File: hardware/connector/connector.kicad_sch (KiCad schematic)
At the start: 16 parts, among them J1 Conn_02x28_Top_Bottom, J2 D38999

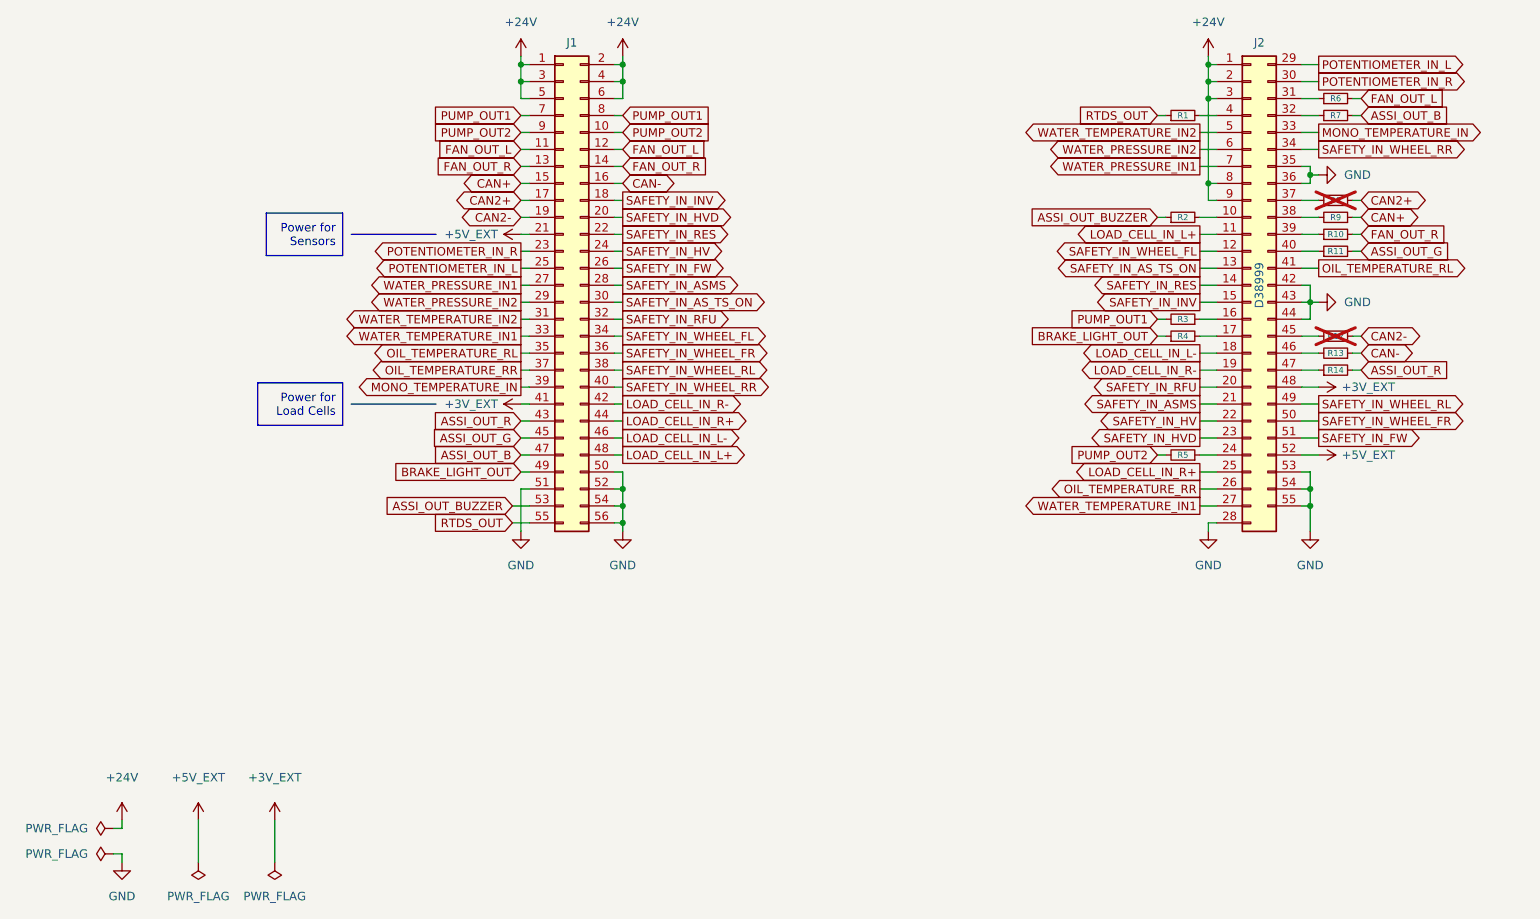
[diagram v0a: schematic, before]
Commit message: Sync :(
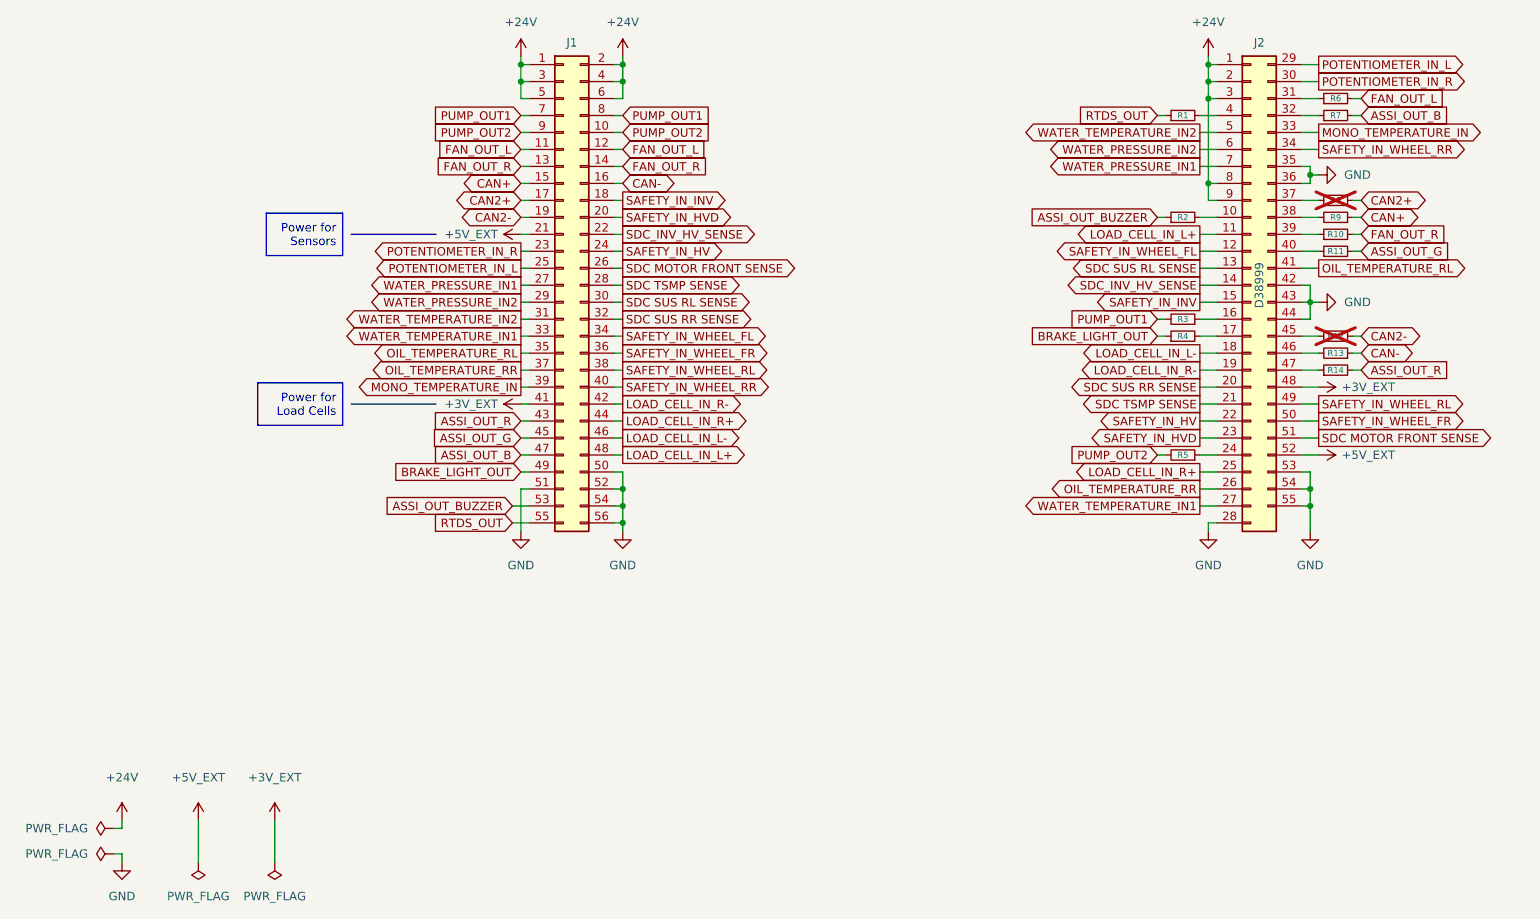
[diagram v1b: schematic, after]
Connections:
- net SAFETY_IN_ASMS renamed SDC TSMP SENSE
- net SAFETY_IN_AS_TS_ON renamed  SDC SUS RL SENSE
- net SAFETY_IN_FW renamed SDC MOTOR FRONT SENSE
- net SAFETY_IN_RES renamed SDC_INV_HV_SENSE
- net SAFETY_IN_RFU renamed  SDC SUS RR SENSE
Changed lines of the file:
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@@
 (kicad_sch
-	(version 20231120)
+	(version 20250114)
 	(generator "eeschema")
-	(generator_version "8.0")
+	(generator_version "9.0")
 	(paper "A4")
 	(title_block
@@
 		(comment 1 "Reviewer:")
 	)
+	(text_box "Power for Sensors"
+		(exclude_from_sim no)
+		(at 59.69 86.995 0)
+		(size 11.43 6.35)
+		(margins 0.9525 0.9525 0.9525 0.9525)
+		(stroke
+			(width 0)
+			(type default)
+		)
+		(fill
+			(type none)
+		)
+		(effects
+			(font
+				(size 1.27 1.27)
+			)
+			(justify right)
+		)
+	)
+	(text_box "Power for Load Cells"
+		(exclude_from_sim no)
+		(at 58.42 112.395 0)
+		(size 12.7 6.35)
+		(margins 0.9525 0.9525 0.9525 0.9525)
+		(stroke
+			(width 0)
+			(type default)
+		)
+		(fill
+			(type none)
+		)
+		(effects
+			(font
+				(size 1.27 1.27)
+			)
+			(justify right)
+		)
+	)
 	(junction
 		(at 113.03 64.77)
@@
 		)
 	)
-	(text_box "Power for Sensors"
-		(exclude_from_sim no)
-		(at 59.69 86.995 0)
-		(size 11.43 6.35)
-		(stroke
-			(width 0)
-			(type default)
-		)
-		(fill
-			(type none)
-		)
-		(effects
-			(font
-				(size 1.27 1.27)
-			)
-			(justify right)
-		)
-	)
-	(text_box "Power for Load Cells"
-		(exclude_from_sim no)
-		(at 58.42 112.395 0)
-		(size 12.7 6.35)
-		(stroke
-			(width 0)
-			(type default)
-		)
-		(fill
-			(type none)
-		)
-		(effects
-			(font
-				(size 1.27 1.27)
-			)
-			(justify right)
-		)
-	)
-	(global_label "SAFETY_IN_RFU"
+	(global_label " SDC SUS RR SENSE"
 		(shape output)
 		(at 113.03 102.87 0)
@@
 		)
 		(property "Intersheetrefs" "${INTERSHEET_REFS}"
-			(at 130.1667 102.87 0)
+			(at 135.9721 102.87 0)
 			(effects
 				(font
@@
 		)
 	)
-	(global_label "SAFETY_IN_ASMS"
+	(global_label "SDC TSMP SENSE"
 		(shape output)
 		(at 199.39 115.57 180)
@@
 		)
 		(property "Intersheetrefs" "${INTERSHEET_REFS}"
-			(at 181.0628 115.57 0)
+			(at 179.7741 115.57 0)
 			(effects
 				(font
@@
 		)
 	)
-	(global_label "SAFETY_IN_AS_TS_ON"
+	(global_label " SDC SUS RL SENSE"
 		(shape output)
 		(at 199.39 95.25 180)
@@
 		)
 		(property "Intersheetrefs" "${INTERSHEET_REFS}"
-			(at 176.871 95.25 0)
+			(at 176.6898 95.25 0)
 			(effects
 				(font
@@
 		)
 	)
-	(global_label "SAFETY_IN_FW"
+	(global_label "SDC MOTOR FRONT SENSE"
 		(shape output)
 		(at 217.17 120.65 0)
@@
 		)
 		(property "Intersheetrefs" "${INTERSHEET_REFS}"
-			(at 233.1576 120.65 0)
+			(at 245.1922 120.65 0)
 			(effects
 				(font
@@
 		)
 	)
-	(global_label "SAFETY_IN_RES"
+	(global_label "SDC_INV_HV_SENSE"
 		(shape output)
 		(at 113.03 90.17 0)
@@
 		)
 		(property "Intersheetrefs" "${INTERSHEET_REFS}"
-			(at 130.0267 90.17 0)
+			(at 134.158 90.17 0)
 			(effects
 				(font
@@
 		)
 	)
-	(global_label "SAFETY_IN_RFU"
+	(global_label " SDC SUS RR SENSE"
 		(shape output)
 		(at 199.39 113.03 180)
@@
 		)
 		(property "Intersheetrefs" "${INTERSHEET_REFS}"
-			(at 182.2533 113.03 0)
+			(at 176.4479 113.03 0)
 			(effects
 				(font
@@
 		)
 	)
-	(global_label "SAFETY_IN_RES"
+	(global_label "SDC_INV_HV_SENSE"
 		(shape output)
 		(at 199.39 97.79 180)
@@
 		)
 		(property "Intersheetrefs" "${INTERSHEET_REFS}"
-			(at 182.3933 97.79 0)
+			(at 178.262 97.79 0)
 			(effects
 				(font
@@
 		)
 	)
-	(global_label "SAFETY_IN_ASMS"
+	(global_label "SDC TSMP SENSE"
 		(shape output)
 		(at 113.03 97.79 0)
@@
 		)
 		(property "Intersheetrefs" "${INTERSHEET_REFS}"
-			(at 131.3572 97.79 0)
+			(at 132.6459 97.79 0)
 			(effects
 				(font
@@
 		)
 	)
-	(global_label "SAFETY_IN_FW"
+	(global_label "SDC MOTOR FRONT SENSE"
 		(shape output)
 		(at 113.03 95.25 0)
@@
 		)
 		(property "Intersheetrefs" "${INTERSHEET_REFS}"
-			(at 128.9382 95.25 0)
+			(at 141.0522 95.25 0)
 			(effects
 				(font
@@
 		)
 	)
-	(global_label "SAFETY_IN_AS_TS_ON"
+	(global_label " SDC SUS RL SENSE"
 		(shape output)
 		(at 113.03 100.33 0)
@@
 		)
 		(property "Intersheetrefs" "${INTERSHEET_REFS}"
-			(at 135.549 100.33 0)
+			(at 135.7302 100.33 0)
 			(effects
 				(font
@@
 		)
 	)
+	(embedded_fonts no)
 )
